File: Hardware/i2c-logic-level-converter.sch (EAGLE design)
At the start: 8 parts, among them Q1 MOSFET-NCHANNELPTH, Q2 MOSFET-NCHANNELPTH

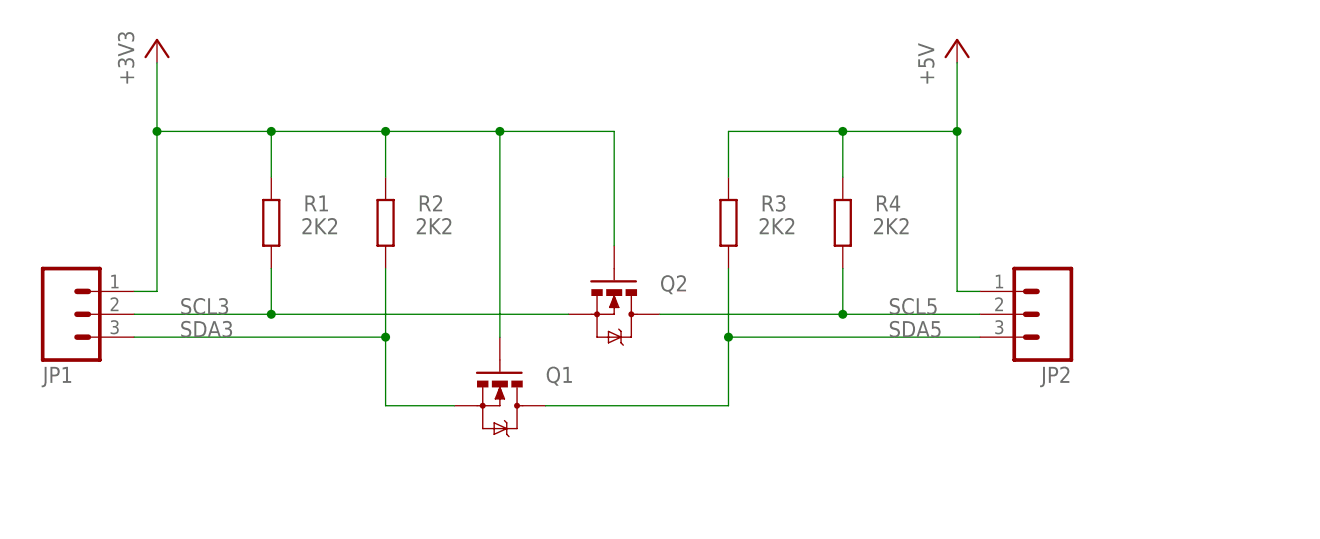
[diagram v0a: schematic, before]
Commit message: rejig Eagle schematic
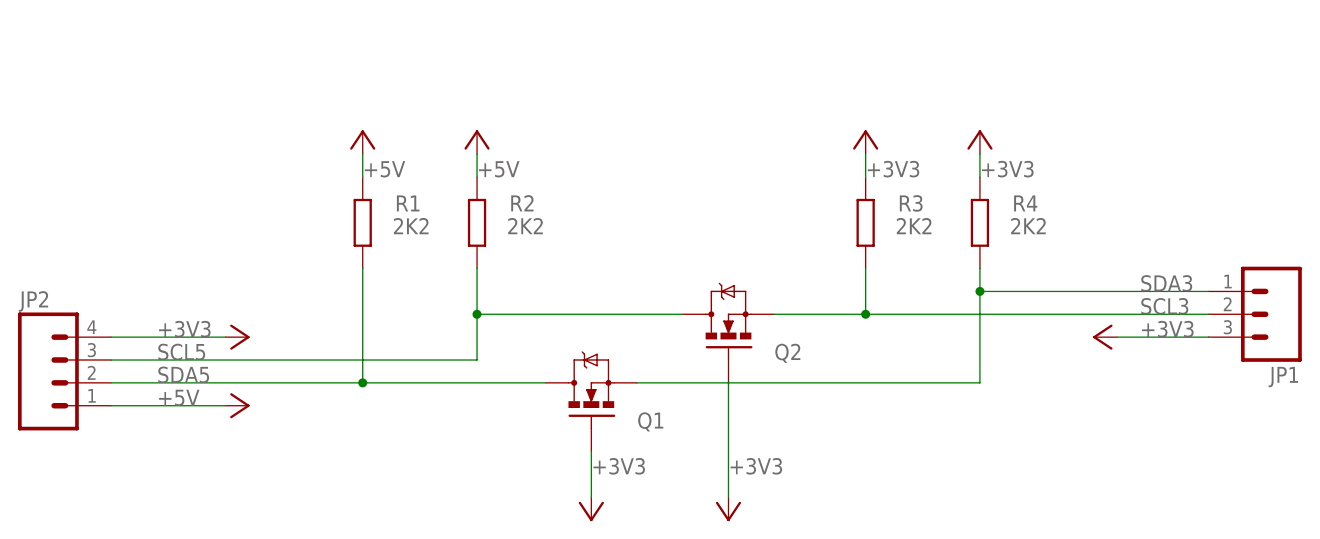
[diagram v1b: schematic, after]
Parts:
- JP2: device SparkFun:M03PTH -> SparkFun:M04PTH
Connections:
- net +3V3: now also JP1.3, JP2.4, R3.2, R4.2; no longer JP1.1, R1.2, R2.2
- net +5V: now also R1.2, R2.2; no longer R3.2, R4.2
- net SCL3: now also R3.1; no longer R1.1
- net SCL5: now also JP2.3, R2.1; no longer JP2.2, R4.1
- net SDA3: now also JP1.1, R4.1; no longer JP1.3, R2.1
- net SDA5: now also JP2.2, R1.1; no longer JP2.3, R3.1
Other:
- moved on the sheet: JP1, Q1, Q2, R1, R2, R3, R4
